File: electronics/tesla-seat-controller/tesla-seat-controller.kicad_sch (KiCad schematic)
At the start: 15 parts, among them J1 USB_C_Receptacle, U1 RP2040, U2 AP63203WU, Y1 ABM8-272-T3

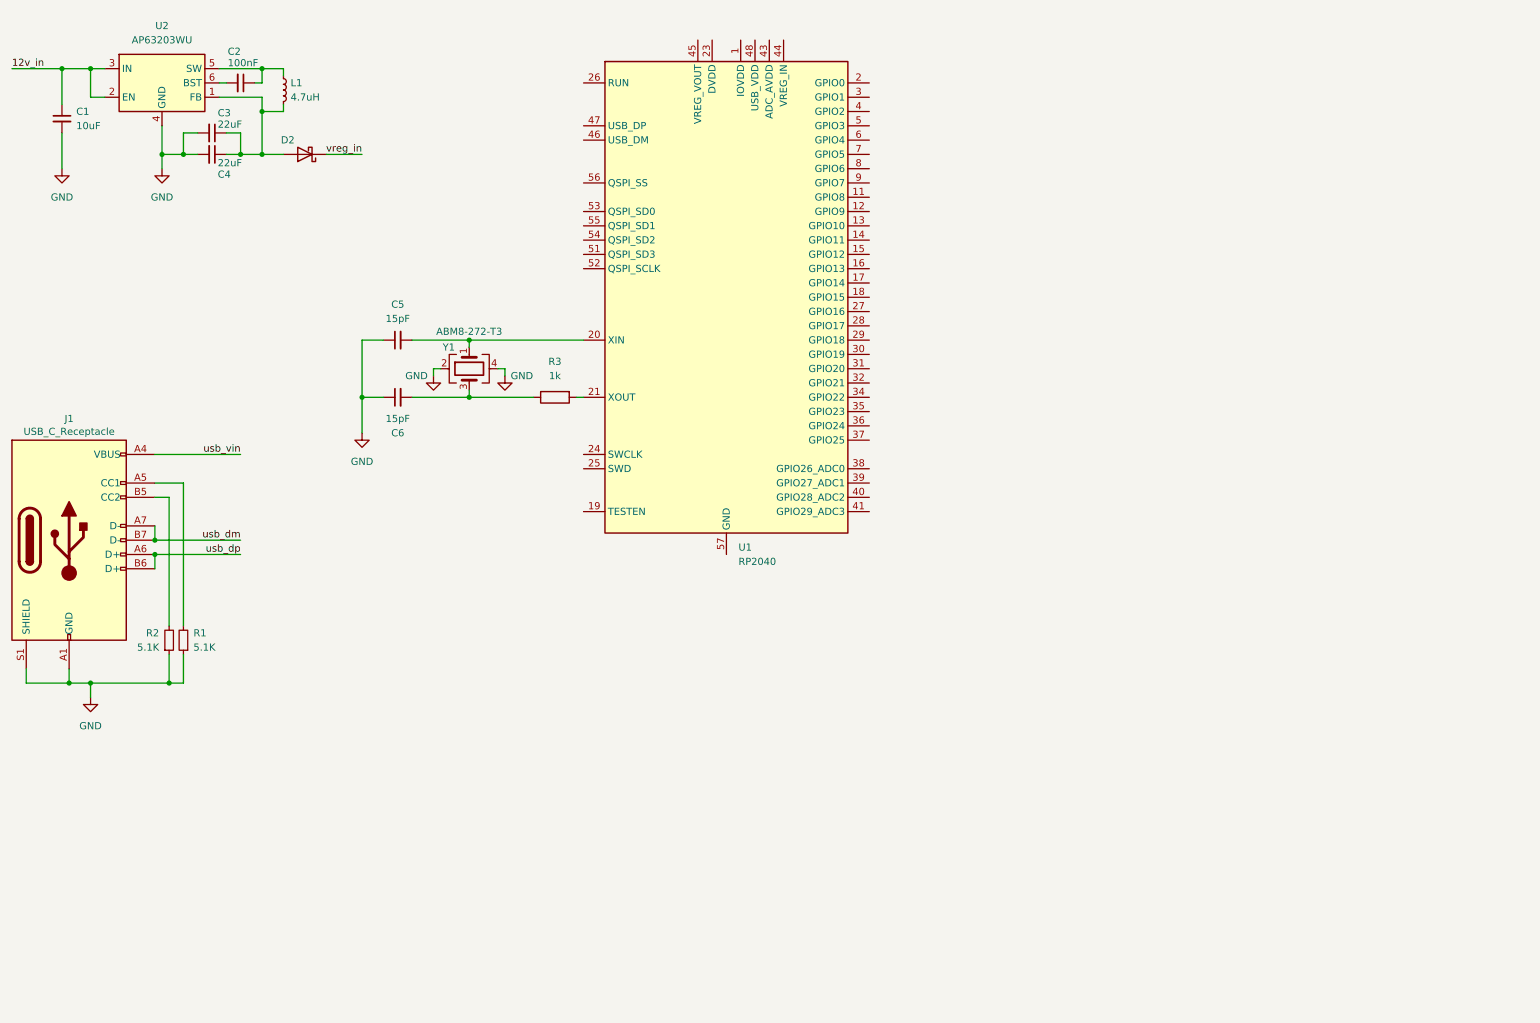
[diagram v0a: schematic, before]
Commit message: update schematic for 2354
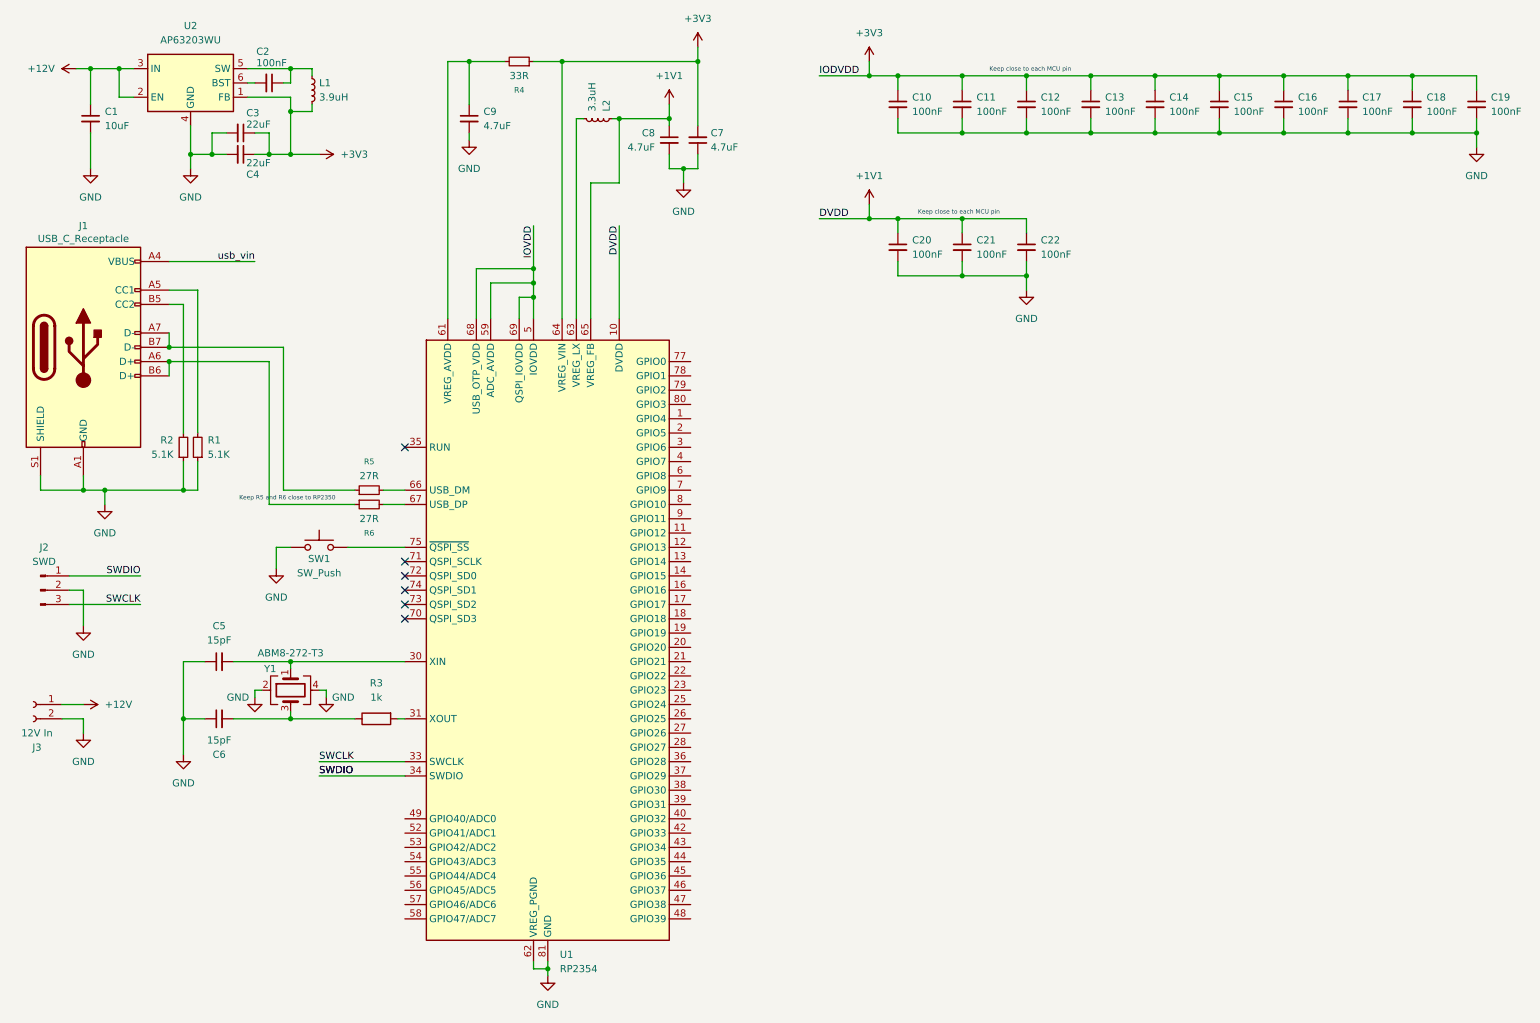
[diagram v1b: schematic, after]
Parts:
- removed D2: D_Schottky, symbol Device:D_Schottky
- added C10, C11, C12, C13, C14, C15, C16, C17, C18, C19, C20, C21, C22: 100nF, symbol Device:C_Small
- added C7, C8, C9: 4.7uF, symbol Device:C_Small
- added J2: SWD, symbol Connector:Conn_01x03_Pin
- added J3: 12V In, symbol Connector:Conn_01x02_Socket
- added L2: 3.3uH, symbol Device:L_Small
- added R4: 33R, symbol Device:R_Small
- added R5, R6: 27R, symbol Device:R_Small
- added SW1: SW_Push, symbol Switch:SW_Push
- L1: value 4.7uH -> 3.9uH
- U1: value RP2040 -> RP2354; footprint Package_DFN_QFN:QFN-56-1EP_7x7mm_P0.4mm_EP3.2x3.2mm -> Package_DFN_QFN:QFN-80-1EP_10x10mm_P0.4mm_EP3.4x3.4mm; symbol MCU_RaspberryPi:RP2040 -> MCU_RaspberryPi:RP2354B
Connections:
- net GND: now also U1.62 (VREG_PGND), U1.81 (GND), C10.2, C11.2, C12.2, C13.2, C14.2, C15.2, C16.2, C17.2, C18.2, C19.2, C20.2, C21.2, C22.2, C7.1, C8.2, C9.2, J2.2 (Pin_2), J3.2 (Pin_2), SW1.2
- net +3V3: now reaches C3.1, C4.1, L1.2, U2.1 (FB)
- net +3V3: now also U1.64 (VREG_VIN), C10.1, C11.1, C12.1, C13.1, C14.1, C15.1, C16.1, C17.1, C18.1, C19.1, C7.2, R4.1
- net at R3.2: now also U1.31 (XOUT); no longer U1.21 (XOUT)
- net at C5.2, Y1.1: now also U1.30 (XIN); no longer U1.20 (XIN)
- net IOVDD: now reaches U1.15 (IOVDD)
- net IOVDD: now also U1.24 (IOVDD), U1.29 (IOVDD), U1.41 (IOVDD), U1.5 (IOVDD), U1.50 (IOVDD), U1.59 (ADC_AVDD), U1.60 (IOVDD), U1.68 (USB_OTP_VDD), U1.69 (QSPI_IOVDD), U1.76 (IOVDD)
- net at U1.23 (GPIO23): no longer U1.50 (DVDD)
- net +1V1: now reaches U1.32 (DVDD)
- net +1V1: now also U1.10 (DVDD), U1.51 (DVDD), U1.65 (VREG_FB), C20.1, C21.1, C22.1, C8.1, L2.2
- net SWDIO: now reaches U1.34 (SWDIO)
- net SWDIO: now also J2.1 (Pin_1)
- net 12v_in renamed +12V
- net +12V: now also J3.1 (Pin_1)
- net usb_dm: no longer names the net of J1.A7 (D-), J1.B7 (D-)
- net usb_dm: now also R5.1
- net usb_dp: no longer names the net of J1.A6 (D+), J1.B6 (D+)
- net usb_dp: now also R6.1
- new net: SW1.1, U1.75 (~{QSPI_SS})
- new net: C9.1, R4.2, U1.61 (VREG_AVDD)
- new net: L2.1, U1.63 (VREG_LX)
- new net: R5.2, U1.66 (USB_DM)
- new net: R6.2, U1.67 (USB_DP)
- new net SWCLK: J2.3 (Pin_3), U1.33 (SWCLK)
- now unconnected: U1.1 (IOVDD), U1.22 (IOVDD), U1.42 (IOVDD), U1.49 (IOVDD)
- no-connect marks 0 -> 6
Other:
- note added: "Keep R5 and R6 close to RP2350"
- note added: "Keep close to each MCU pin"
- moved on the sheet: C1, C2, C3, C4, C5, C6, J1, L1, R1, R2, R3, U2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
